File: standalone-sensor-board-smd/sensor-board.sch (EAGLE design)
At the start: 15 parts, among them Q1 QRE1113, Q2 QRE1113, Q3 QRE1113, Q4 QRE1113, Q5 QRE1113, Q6 QRE1113, Q7 QRE1113

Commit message: init smd
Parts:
- Q1, Q2, Q3, Q4, Q5, Q6, Q7: value QRE1113 -> QRE1113GR; device qre1113:QRE1113 -> qre1113:QRE1113GR
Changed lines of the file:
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@@
 </classes>
 <parts>
-<part name="Q1" library="qre1113" deviceset="QRE1113" device=""/>
+<part name="Q1" library="qre1113" deviceset="QRE1113GR" device=""/>
 <part name="R1" library="rcl" library_urn="urn:adsk.eagle:library:334" deviceset="R-EU_" device="0204/2V" package3d_urn="urn:adsk.eagle:package:23495/1" value="100"/>
-<part name="Q2" library="qre1113" deviceset="QRE1113" device=""/>
+<part name="Q2" library="qre1113" deviceset="QRE1113GR" device=""/>
 <part name="R3" library="rcl" library_urn="urn:adsk.eagle:library:334" deviceset="R-EU_" device="0204/2V" package3d_urn="urn:adsk.eagle:package:23495/1" value="100"/>
-<part name="Q3" library="qre1113" deviceset="QRE1113" device=""/>
+<part name="Q3" library="qre1113" deviceset="QRE1113GR" device=""/>
 <part name="R5" library="rcl" library_urn="urn:adsk.eagle:library:334" deviceset="R-EU_" device="0204/2V" package3d_urn="urn:adsk.eagle:package:23495/1" value="100"/>
-<part name="Q4" library="qre1113" deviceset="QRE1113" device=""/>
+<part name="Q4" library="qre1113" deviceset="QRE1113GR" device=""/>
 <part name="R7" library="rcl" library_urn="urn:adsk.eagle:library:334" deviceset="R-EU_" device="0204/2V" package3d_urn="urn:adsk.eagle:package:23495/1" value="100"/>
-<part name="Q5" library="qre1113" deviceset="QRE1113" device=""/>
+<part name="Q5" library="qre1113" deviceset="QRE1113GR" device=""/>
 <part name="R9" library="rcl" library_urn="urn:adsk.eagle:library:334" deviceset="R-EU_" device="0204/2V" package3d_urn="urn:adsk.eagle:package:23495/1" value="100"/>
-<part name="Q6" library="qre1113" deviceset="QRE1113" device=""/>
+<part name="Q6" library="qre1113" deviceset="QRE1113GR" device=""/>
 <part name="R11" library="rcl" library_urn="urn:adsk.eagle:library:334" deviceset="R-EU_" device="0204/2V" package3d_urn="urn:adsk.eagle:package:23495/1" value="100"/>
-<part name="Q7" library="qre1113" deviceset="QRE1113" device=""/>
+<part name="Q7" library="qre1113" deviceset="QRE1113GR" device=""/>
 <part name="R13" library="rcl" library_urn="urn:adsk.eagle:library:334" deviceset="R-EU_" device="0204/2V" package3d_urn="urn:adsk.eagle:package:23495/1" value="100"/>
 <part name="SUPPLY7" library="supply2" library_urn="urn:adsk.eagle:library:372" deviceset="VCC" device=""/>

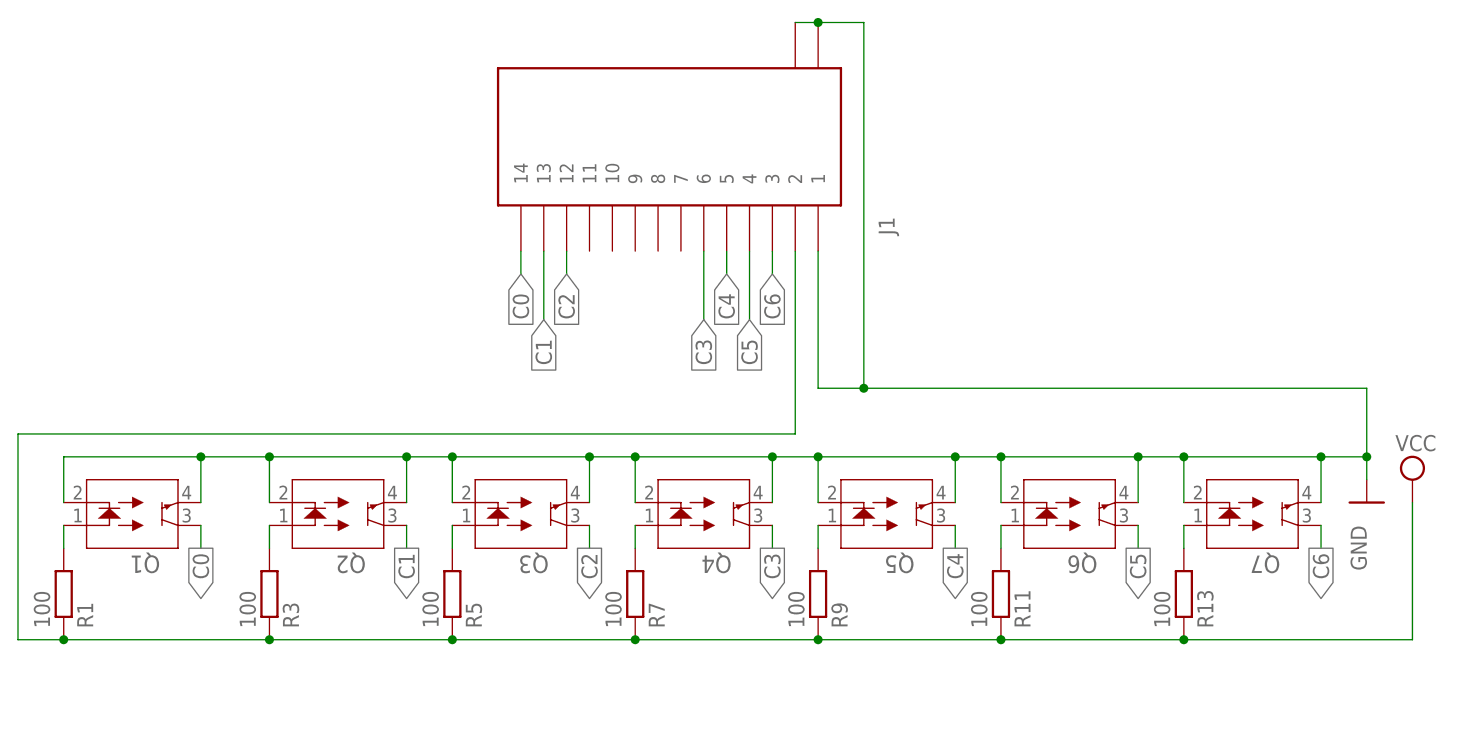
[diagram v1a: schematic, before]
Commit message: add smd boards from standalone
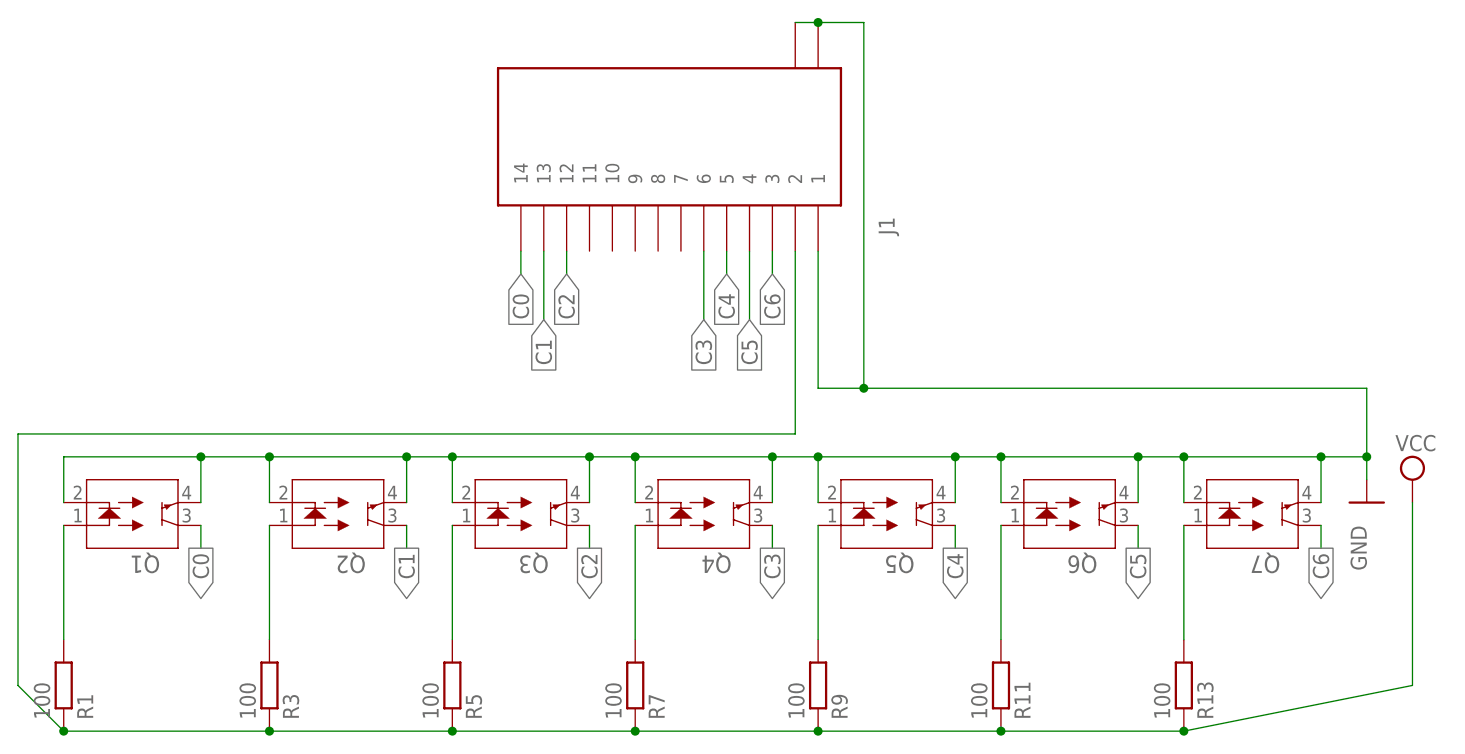
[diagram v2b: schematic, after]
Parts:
- Q1, Q2, Q3, Q4, Q5, Q6, Q7: value QRE1113GR -> QRE1113; device qre1113:QRE1113GR -> qre1113:QRE1113
- R1, R11, R13, R3, R5, R7, R9: device rcl:R-EU_0204/2V -> rcl:R-EU_R0805
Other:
- moved on the sheet: R1, R11, R13, R3, R5, R7, R9
